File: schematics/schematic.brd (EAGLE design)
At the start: 125 x 93 mm, 55 parts, among them IC1 74HC365, T1 BC547, X5 PN61729-S

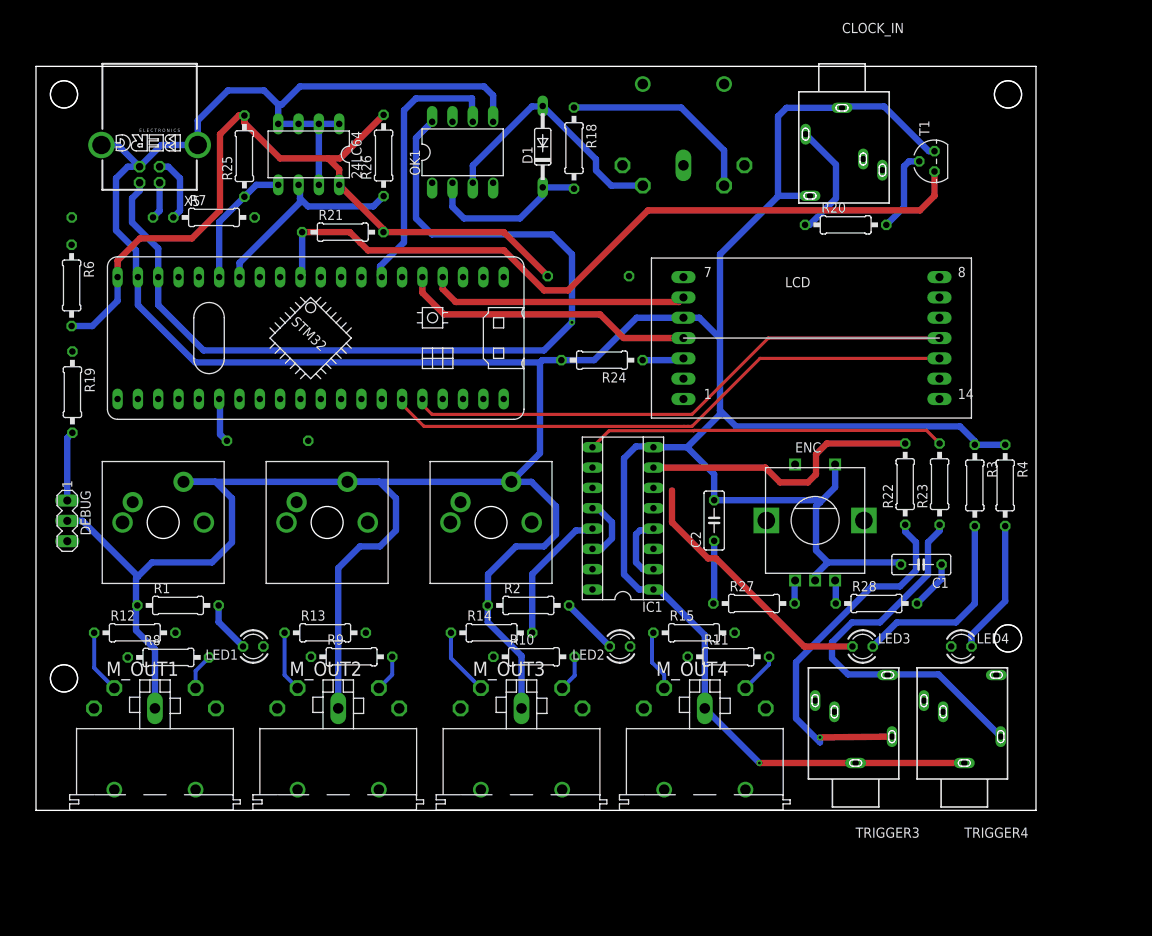
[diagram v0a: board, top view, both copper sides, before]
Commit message: finished first version of schematic;
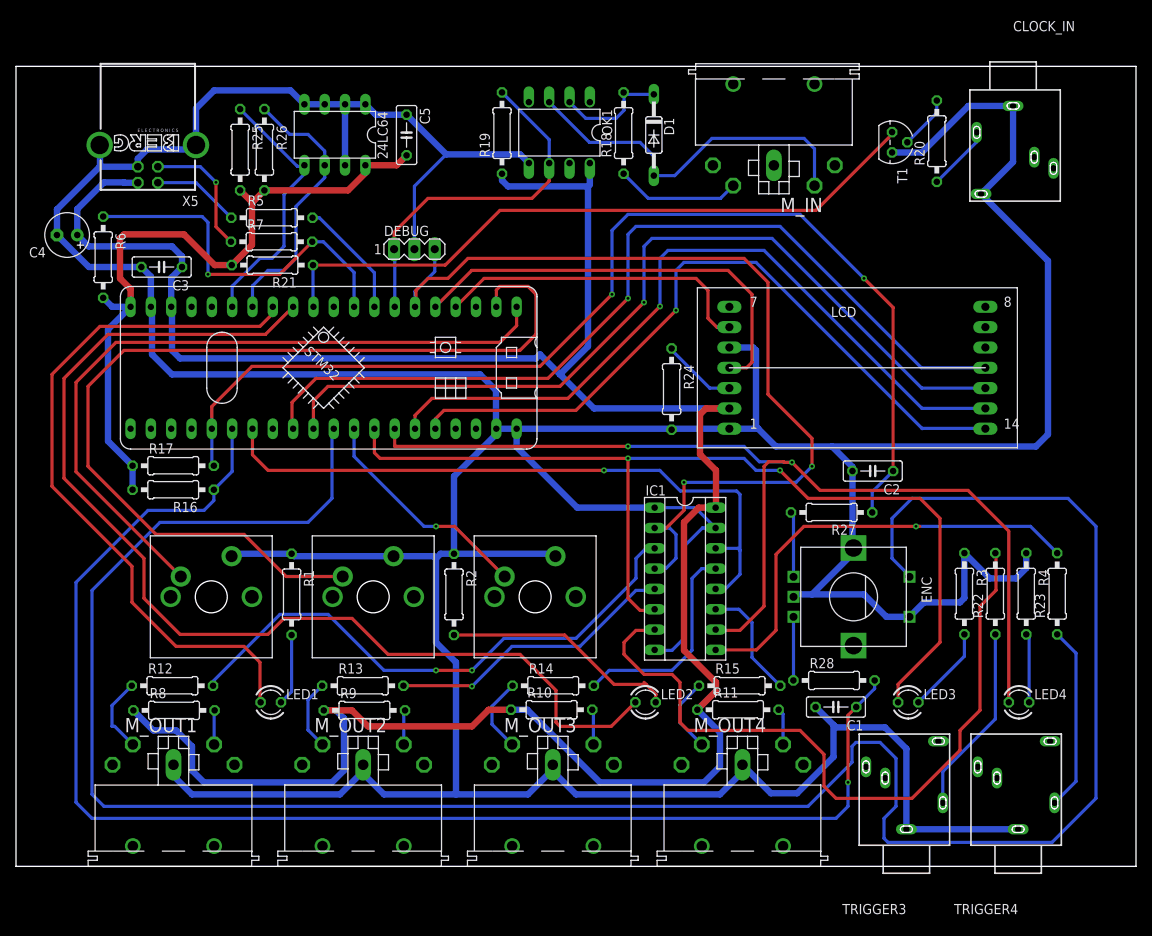
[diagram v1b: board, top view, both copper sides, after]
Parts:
- added C3, C5: 0.1 uF, rcl:C050-025X075
- added C4: 10uF, rcl:E2,5-6
- moved R19 62.7 mm to (60.8, 91.7), turned to 90 degrees
- moved R17 57.1 mm to (19.6, 50.1), flipped to the top, turned to 0 degrees
- moved DEBUG 55.1 mm to (49.8, 77.2), turned to 0 degrees
- moved CLOCK_IN 21.4 mm to (124.6, 97.2)
- moved C2 20.8 mm to (107.1, 49.4), turned to 180 degrees
- moved C1 20.8 mm to (102.5, 19.9)
- moved R23 20.1 mm to (130.1, 34.1)
- moved R5 19.9 mm to (32.0, 81.1), flipped to the top
- moved R22 17.7 mm to (122.4, 34.1)
- moved R20 15.5 mm to (115.1, 90.7), turned to 90 degrees
- moved R27 15.0 mm to (102.0, 44.2), turned to 180 degrees
- moved R26 14.9 mm to (31.0, 89.6), turned to 270 degrees
- moved R1 14.3 mm to (34.5, 34.0), turned to 270 degrees
- moved D1 14.0 mm to (79.7, 91.4), turned to 270 degrees
- moved R4 13.8 mm to (126.3, 34.1)
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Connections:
- removed net GND1: STM32F103.P$21
- net +3V3: now also C5.2
- net +5V: now also C3.1, C4.+
- net GND: now also C3.2, C4.-, C5.1, STM32F103.P$21, STM32F103.P$22
- net PA4: now also LCD.11; no longer LCD.13
- net PA5: now also LCD.12; no longer LCD.14
- net PB10: now also LCD.13; no longer LCD.12
- net PB11: now also LCD.14; no longer LCD.11
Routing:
- net PA6: track 0.00 -> 285.3 mm
- net +5V: track 115.3 -> 304.9 mm, vias 1 -> 0
- net PA1: track 11.8 -> 174.0 mm, vias 0 -> 1
- net PB4: track 0.00 -> 137.3 mm
- net PB1: track 0.00 -> 133.4 mm, vias 0 -> 2
- net PA0: track 7.87 -> 138.8 mm, vias 0 -> 2
- net PB13: track 0.00 -> 118.9 mm
- net PA4: track 0.00 -> 111.1 mm, vias 0 -> 1
- net PA9: track 8.51 -> 116.8 mm, vias 0 -> 2
- net PA5: track 0.00 -> 107.7 mm, vias 0 -> 1
- net PB0: track 33.0 -> 123.8 mm, vias 0 -> 2
- net PB12: track 0.00 -> 90.1 mm
- net PB5: track 0.00 -> 88.8 mm
- net PA2: track 8.16 -> 84.8 mm, vias 0 -> 1
- net N$17: track 0.00 -> 69.9 mm, vias 0 -> 2
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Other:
- board size 125 x 93 mm -> 140 x 100 mm
